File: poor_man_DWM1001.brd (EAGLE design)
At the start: 32.6 x 26 mm, 18 parts, among them CN1 B2B-PH-K-S, IC1 E73_2G4M04S, U1 DWM1000_BREAKOUT, U3 MIC5205-3.3YM5-TR

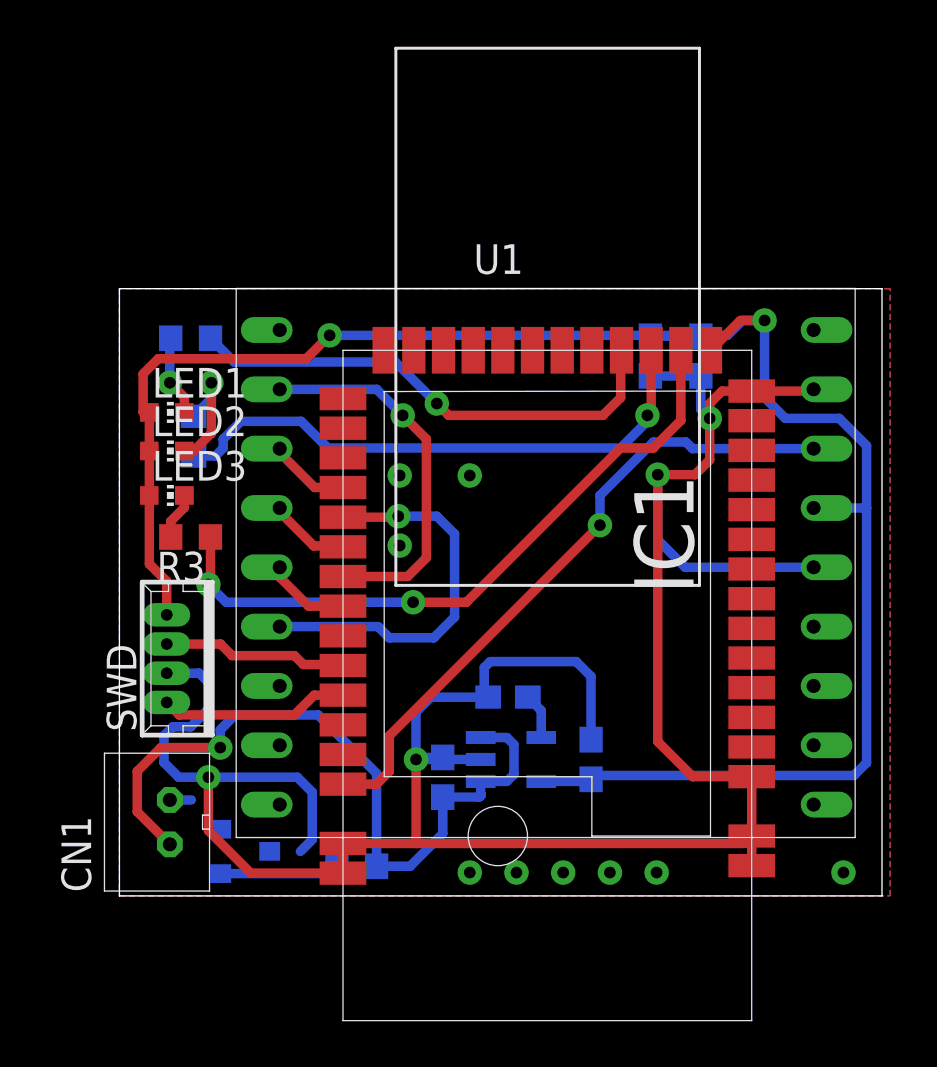
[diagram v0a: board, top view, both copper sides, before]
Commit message: Daily save
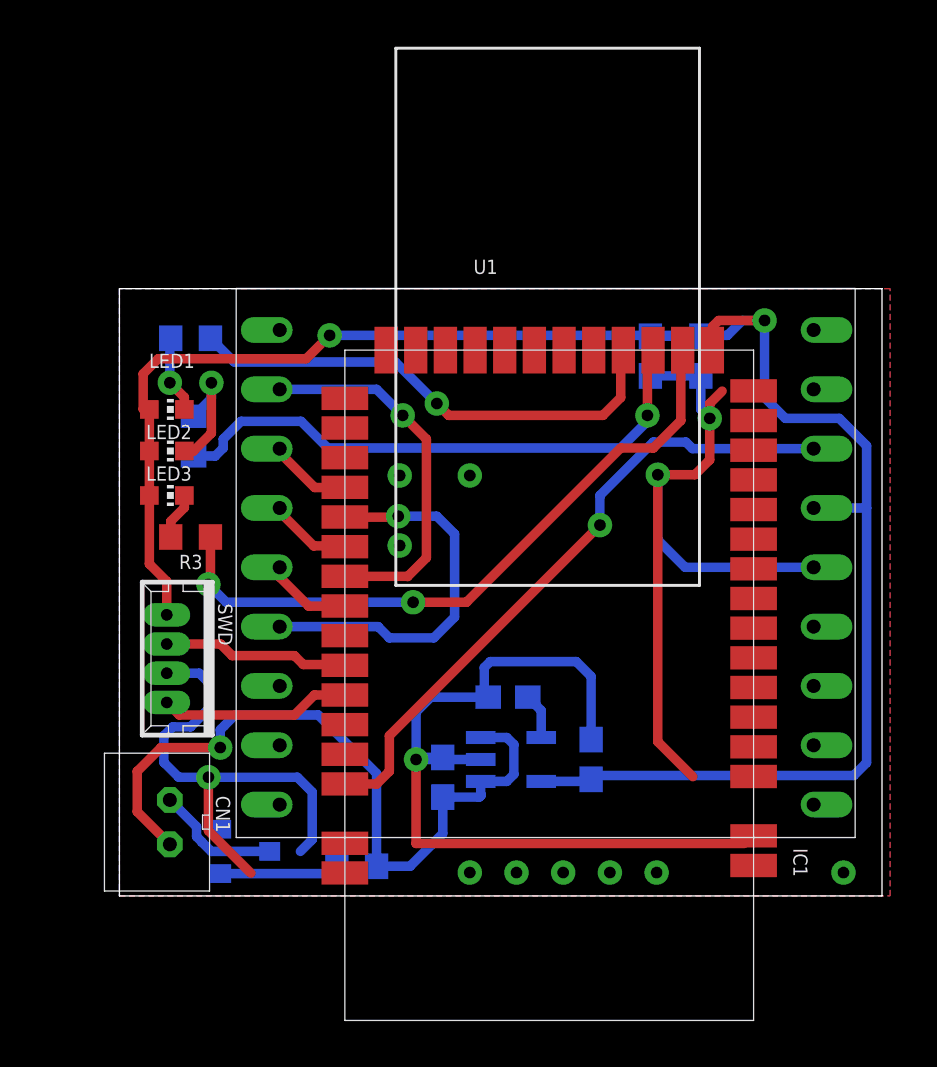
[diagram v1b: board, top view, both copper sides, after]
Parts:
- moved LED1 0.13 mm to (2.03, 20.8)
- moved IC1 0.08 mm to (9.65, 23.4)
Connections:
- net DEC5 renamed DEC1
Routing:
- net GND: track 109.8 -> 90.8 mm
- net AGND: track 0.92 -> 5.44 mm
- net +3V3: track 82.4 -> 82.9 mm
